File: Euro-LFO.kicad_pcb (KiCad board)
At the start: 2 copper layers, 81 x 128.5 mm, 40 parts, among them J1 2×5 2.54 mm shrouded IDC box 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, J3 Conn_01x07_Socket, J4 Conn_01x07_Pin, J5 Conn_01x07_Socket, J6 Conn_01x07_Pin, Q1 MMBT3904, U1 TL074CDR

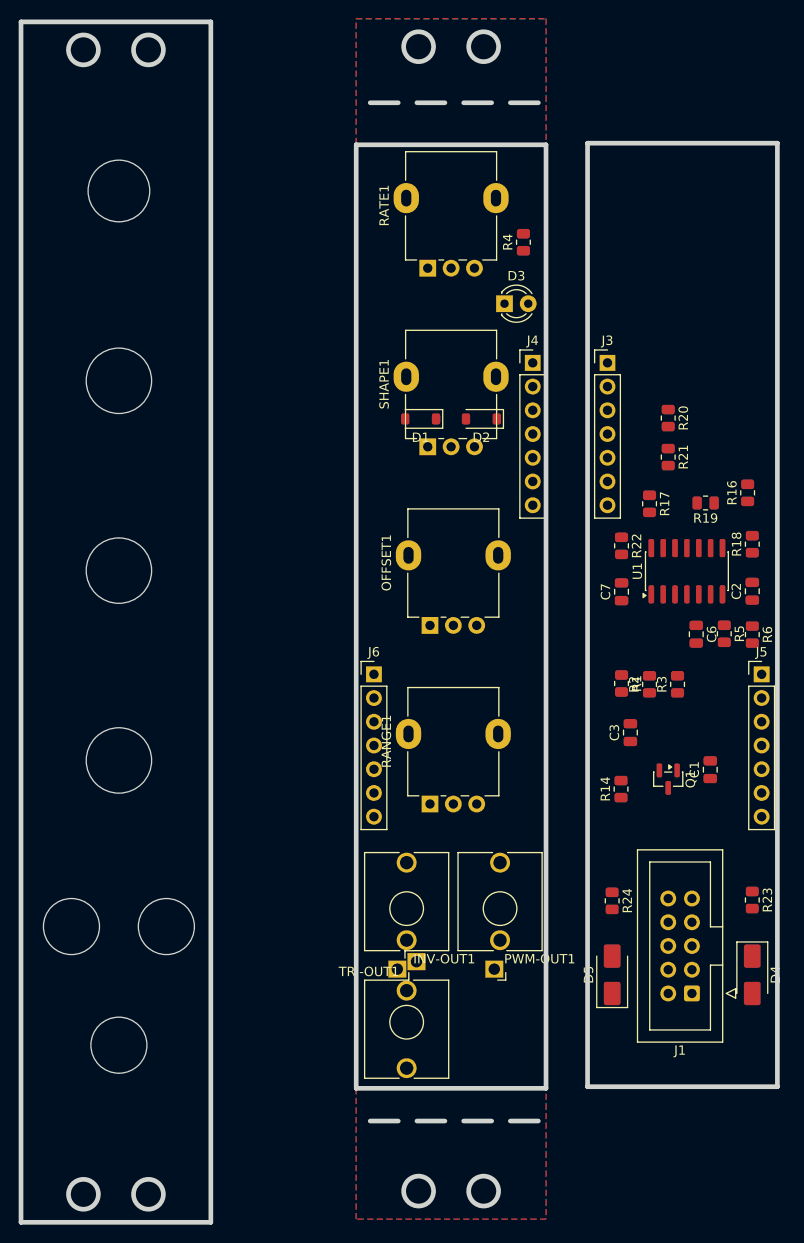
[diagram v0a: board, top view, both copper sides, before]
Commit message: work in progress
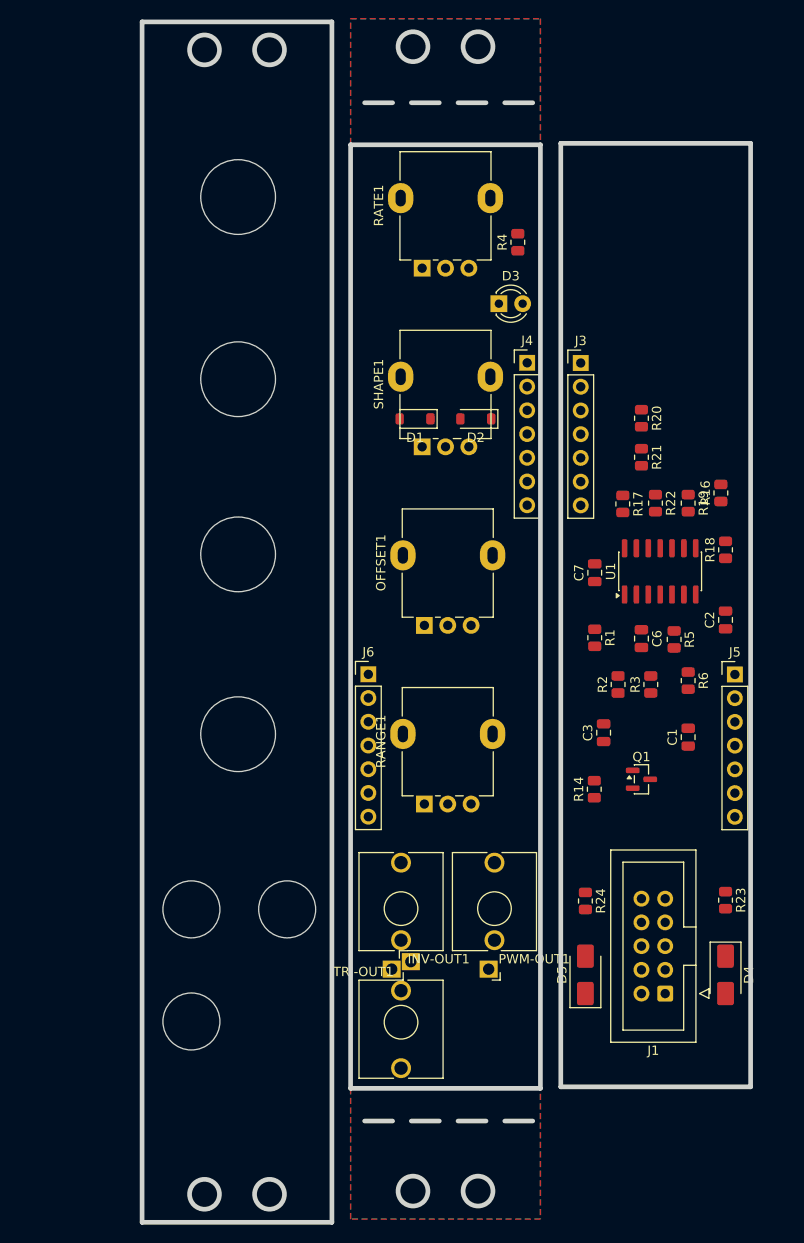
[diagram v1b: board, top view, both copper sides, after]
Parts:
- moved R6 8.45 mm to (137.1, 90.5)
- moved C6 5.88 mm to (132.1, 86.0)
- moved R22 5.84 mm to (133.6, 71.5)
- moved R1 5.67 mm to (127.1, 85.9)
- moved R5 5.40 mm to (135.6, 86.1)
- moved C1 4.21 mm to (137.1, 96.6)
- moved C2 4.20 mm to (141.1, 84.0)
- moved C7 3.51 mm to (127.1, 79.0)
- moved R2 3.37 mm to (129.6, 90.9)
- moved R18 2.93 mm to (141.1, 76.5)
- moved D4 2.87 mm to (141.1, 122.0)
- moved J5 2.87 mm to (142.1, 89.9)
- moved Q1 2.87 mm to (132.1, 101.1), turned to 0 degrees
- moved R16 2.87 mm to (140.6, 70.4)
- moved R17 2.87 mm to (130.1, 71.6)
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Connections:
- J5 pad 5: unconnected-(J5-Pin_5-Pad5) -> /U1A_I
- J6 pad 5: unconnected-(J6-Pin_5-Pad5) -> /U1A_O
- R1 pad 2: /U!A_I -> /U1A_I
- R2 pad 2: /U!A_I -> /U1A_I
- U1 pad 1: /U!A_I -> /U1A_I
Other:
- board size 81 x 128.5 mm -> 65.1 x 128.5 mm

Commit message: Sorting out cross board connections
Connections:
- J5 pad 1: +12V -> /U1A_I
- J5 pad 2: /OFF_I -> +12V
- J5 pad 3: /RNG_3_I -> /OFF_I
- J5 pad 4: /RNG_2_I -> -12V
- J5 pad 5: /U1A_I -> /RNG_3_I
- J5 pad 6: unconnected-(J5-Pin_6-Pad6) -> /RNG_2_I
- J5 pad 7: -12V -> unconnected-(J5-Pin_7-Pad7)
- J6 pad 1: /+12_O -> /U1A_O
- J6 pad 2: /OFF_O -> /+12_O
- J6 pad 3: /RNG_3_O -> /OFF_O
- J6 pad 4: /RNG_2_O -> /-12_O
- J6 pad 5: /U1A_O -> /RNG_3_O
- J6 pad 6: unconnected-(J6-Pin_6-Pad6) -> /RNG_2_O
- J6 pad 7: /-12_O -> unconnected-(J6-Pin_7-Pad7)
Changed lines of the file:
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@@
 			(layers "*.Cu" "*.Mask")
 			(remove_unused_layers no)
-			(net "/+12_O")
+			(net "/U1A_O")
 			(pinfunction "Pin_1_1")
 			(pintype "passive")
@@
 			(layers "*.Cu" "*.Mask")
 			(remove_unused_layers no)
-			(net "/OFF_O")
+			(net "/+12_O")
 			(pinfunction "Pin_2_2")
 			(pintype "passive")
@@
 			(layers "*.Cu" "*.Mask")
 			(remove_unused_layers no)
-			(net "/RNG_3_O")
+			(net "/OFF_O")
 			(pinfunction "Pin_3_3")
 			(pintype "passive")
@@
 			(layers "*.Cu" "*.Mask")
 			(remove_unused_layers no)
-			(net "/RNG_2_O")
+			(net "/-12_O")
 			(pinfunction "Pin_4_4")
 			(pintype "passive")
@@
 			(layers "*.Cu" "*.Mask")
 			(remove_unused_layers no)
-			(net "/U1A_O")
+			(net "/RNG_3_O")
 			(pinfunction "Pin_5_5")
 			(pintype "passive")
@@
 			(layers "*.Cu" "*.Mask")
 			(remove_unused_layers no)
-			(net "unconnected-(J6-Pin_6-Pad6)")
+			(net "/RNG_2_O")
 			(pinfunction "Pin_6_6")
 			(pintype "passive")
@@
 			(layers "*.Cu" "*.Mask")
 			(remove_unused_layers no)
-			(net "/-12_O")
+			(net "unconnected-(J6-Pin_7-Pad7)")
 			(pinfunction "Pin_7_7")
 			(pintype "passive")
@@
 			(layers "*.Cu" "*.Mask")
 			(remove_unused_layers no)
-			(net "+12V")
+			(net "/U1A_I")
 			(pinfunction "Pin_1_1")
 			(pintype "passive")
@@
 			(layers "*.Cu" "*.Mask")
 			(remove_unused_layers no)
-			(net "/OFF_I")
+			(net "+12V")
 			(pinfunction "Pin_2_2")
 			(pintype "passive")
@@
 			(layers "*.Cu" "*.Mask")
 			(remove_unused_layers no)
-			(net "/RNG_3_I")
+			(net "/OFF_I")
 			(pinfunction "Pin_3_3")
 			(pintype "passive")
@@
 			(layers "*.Cu" "*.Mask")
 			(remove_unused_layers no)
-			(net "/RNG_2_I")
+			(net "-12V")
 			(pinfunction "Pin_4_4")
 			(pintype "passive")
@@
 			(layers "*.Cu" "*.Mask")
 			(remove_unused_layers no)
-			(net "/U1A_I")
+			(net "/RNG_3_I")
 			(pinfunction "Pin_5_5")
 			(pintype "passive")
@@
 			(layers "*.Cu" "*.Mask")
 			(remove_unused_layers no)
-			(net "unconnected-(J5-Pin_6-Pad6)")
+			(net "/RNG_2_I")
 			(pinfunction "Pin_6_6")
 			(pintype "passive")
@@
 			(layers "*.Cu" "*.Mask")
 			(remove_unused_layers no)
-			(net "-12V")
+			(net "unconnected-(J5-Pin_7-Pad7)")
 			(pinfunction "Pin_7_7")
 			(pintype "passive")
